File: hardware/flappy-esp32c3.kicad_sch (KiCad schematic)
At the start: 55 parts, among them J1 USB-C-Breakout 16P, J2 LiPo 1S 500 mAh, J3 OLED SSD1306 SPI, J4 Arcade-Taster, SW1 Ein/Aus, U1 ESP32-C3-WROOM-02-N4, U2 MCP73831-2-OT, U3 AP2112K-3.3

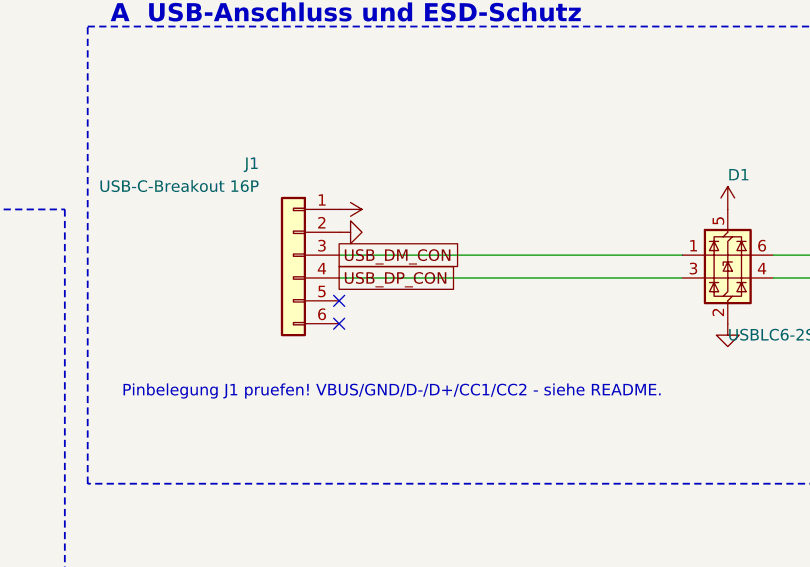
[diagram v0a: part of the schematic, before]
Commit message: update
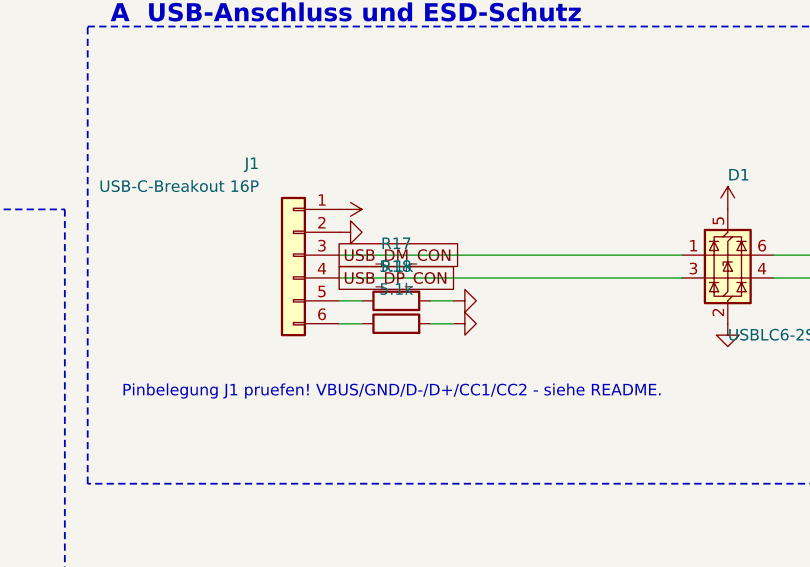
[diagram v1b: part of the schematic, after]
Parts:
- added R17, R18: 5.1k, Resistor_SMD:R_0805_2012Metric_Pad1.20x1.40mm_HandSolder, symbol Device:R
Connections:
- net GND: now also R17.2, R18.2
- net at J1.5 (Pin_5): now also R17.1
- net at J1.6 (Pin_6): now also R18.1
- no-connect marks 7 -> 5

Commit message: update
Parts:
- removed LS1: Piezo 12 mm, Buzzer_Beeper:Buzzer_12x9.5RM7.6, symbol Device:Buzzer
- added J5: Piezo CEP-1114, Connector_JST:JST_XH_B2B-XH-A_1x02_P2.50mm_Vertical, symbol Connector_Generic:Conn_01x02
- C1: value 4u7 -> 4u7 25V X7R
- C10, C11, C2, C4, C7, C9: value 100n -> 100n 50V X7R
- C3: value 4u7 -> 10u 25V X7R
- C5: value 1u -> 2u2 16V X7R
- C6: value 22u -> 22u 10V X5R
- C8: value 10u -> 10u 16V X7R
- R14: value 1k -> 330R
- R17, R18: value 5.1k -> 5k1; now not fitted
- R2: value 1k -> 560R
- U2: value MCP73831-2-OT -> MCP73831T-2ACI/OT
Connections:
- net BUZZ_P: now also J5.1 (Pin_1)
- net GND: now also J5.2 (Pin_2)
- net USB_CC1: now reaches J1.5 (Pin_5), R17.1
- net USB_CC2: now reaches J1.6 (Pin_6), R18.1
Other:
- note added: "2,55 k an CC bei 80 uA nur 0,204 V - Totzone zwischen vRa und vRd-Connect."
- note added: "Beleg fuer D3 fehlt (K-4): das echte B5819W-Datenblatt ist noch abzulegen."
- note added: "C6 = 22u/10V X5R + C8 = 10u/16V X7R stuetzen die Sendespitze. Wirksame"
- note added: "H Tonausgabe (JST-XH 2-polig), Betriebsanzeige, Pruefpunkte"
- note added: "Kapazitaet bei 3,3 V DC-Bias im Datenblatt des gewaehlten Typs pruefen (K-3):"
- note added: "LS1 (CEP-1114) ist D30 mm / RM 20 mm und sitzt abgesetzt am Kabel an J5 (K-1)."
- note added: "R13 begrenzt den GPIO-Strom auf 3,3 V / 220 R = 15 mA; C_Piezo = 45 nF typ."
- note added: "R14 = 330 R -> 4,1 mA: die GaP-Gruene ist bei 1,3 mA praktisch unsichtbar (M-9)."
- note added: "R17/R18 ab Werk NICHT bestueckt (K-2): hat das Breakout eigene 5k1, ergeben"
- note added: "nominell 32 uF, derated eher 15..18 uF -> Droop 350 mA * 10 us / 16 uF = 220 mV."
- note removed: "C6 = 22 uF stuetzt die Sendespitze: 350 mA * 10 us / 100 mV = 35 uF (5.4),"
- note removed: "H Tonausgabe, Betriebsanzeige, Pruefpunkte"
- note removed: "zusammen mit C8 = 10 uF unmittelbar am Modul. X5R-Derating beachten."

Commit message: .
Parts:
- added C12: 100n 50V X7R, Capacitor_SMD:C_0805_2012Metric_Pad1.18x1.45mm_HandSolder, symbol Device:C
- added D5: USBLC6-2SC6, Package_TO_SOT_SMD:SOT-23-6_Handsoldering, symbol Power_Protection:USBLC6-2SC6
- added R19, R22, R23: 1M, Resistor_SMD:R_0805_2012Metric_Pad1.20x1.40mm_HandSolder, symbol Device:R
- added R20, R21: 100k, Resistor_SMD:R_0805_2012Metric_Pad1.20x1.40mm_HandSolder, symbol Device:R
- J3: footprint Connector_JST:JST_XH_B7B-XH-A_1x07_P2.50mm_Vertical -> Connector_JST:JST_XH_B8B-XH-A_1x08_P2.50mm_Vertical; symbol Connector_Generic:Conn_01x07 -> Connector_Generic:Conn_01x08
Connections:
- net +3V3_MCU: now also D5.5 (VBUS)
- net BTN_CON: now also D5.1 (I/O1), D5.6 (I/O1)
- net BUZZ_P: now also D5.3 (I/O2), D5.4 (I/O2)
- net GND: now also J3.4 (Pin_4), C12.2, D5.2 (GND), R19.2, R21.2, R23.2
- net LED_G: now also U1.10 (IO10); no longer U1.18 (IO0)
- net MOSI: now also J3.5 (Pin_5); no longer J3.4 (Pin_4)
- net OLED_CS: now also J3.8 (Pin_8); no longer J3.7 (Pin_7)
- net OLED_DC: now also J3.7 (Pin_7); no longer J3.6 (Pin_6)
- net OLED_RES: now also J3.6 (Pin_6); no longer J3.5 (Pin_5)
- net VBAT: now also C5.1, U3.1 (VIN), R22.1
- net VBUS: now also R20.1
- net VBUS_SENSE: now reaches U1.11 (IO20/RXD)
- net VBUS_SENSE: now also R20.2, R21.1
- net VBAT_SW renamed LDO_EN
- net LDO_EN: now also R19.1; no longer C5.1, U3.1 (VIN)
- new net VBAT_SENSE: C12.1, R22.2, R23.1, U1.18 (IO0)
- no-connect marks 5 -> 3
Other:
- note added: "M-5: SW1 schaltet nur noch EN. Kontaktstrom 4,2 V / 750 k = 5,6 uA statt 345 mA."
- note added: "M-6: VBUS-Teiler an IO20 - die Firmware erkennt USB und kann die Last senken,"
- note added: "M-8/M-10: D5 klemmt beide Kabeladern auf GND und +3V3_MCU. Ohne sie schlaegt"
- note added: "R12 bei 8 kV mit 2708 V ueber, und der Piezo speist 103 mA in IO1 zurueck."
- note added: "bis I < I_TERM = 11 mA. Erst dann terminiert der Ladevorgang (kein 4,2-V-Dauerfloat)."
- note removed: "Keine Lastpfadumschaltung: zum Laden wird das Geraet ausgeschaltet (4.1)."
- note removed: "U3 EN fest auf VBAT_SW: der Schiebeschalter schaltet die gesamte Versorgung."
